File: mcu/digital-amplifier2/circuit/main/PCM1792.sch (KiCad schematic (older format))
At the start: 16 parts, among them U12 PCM1792A

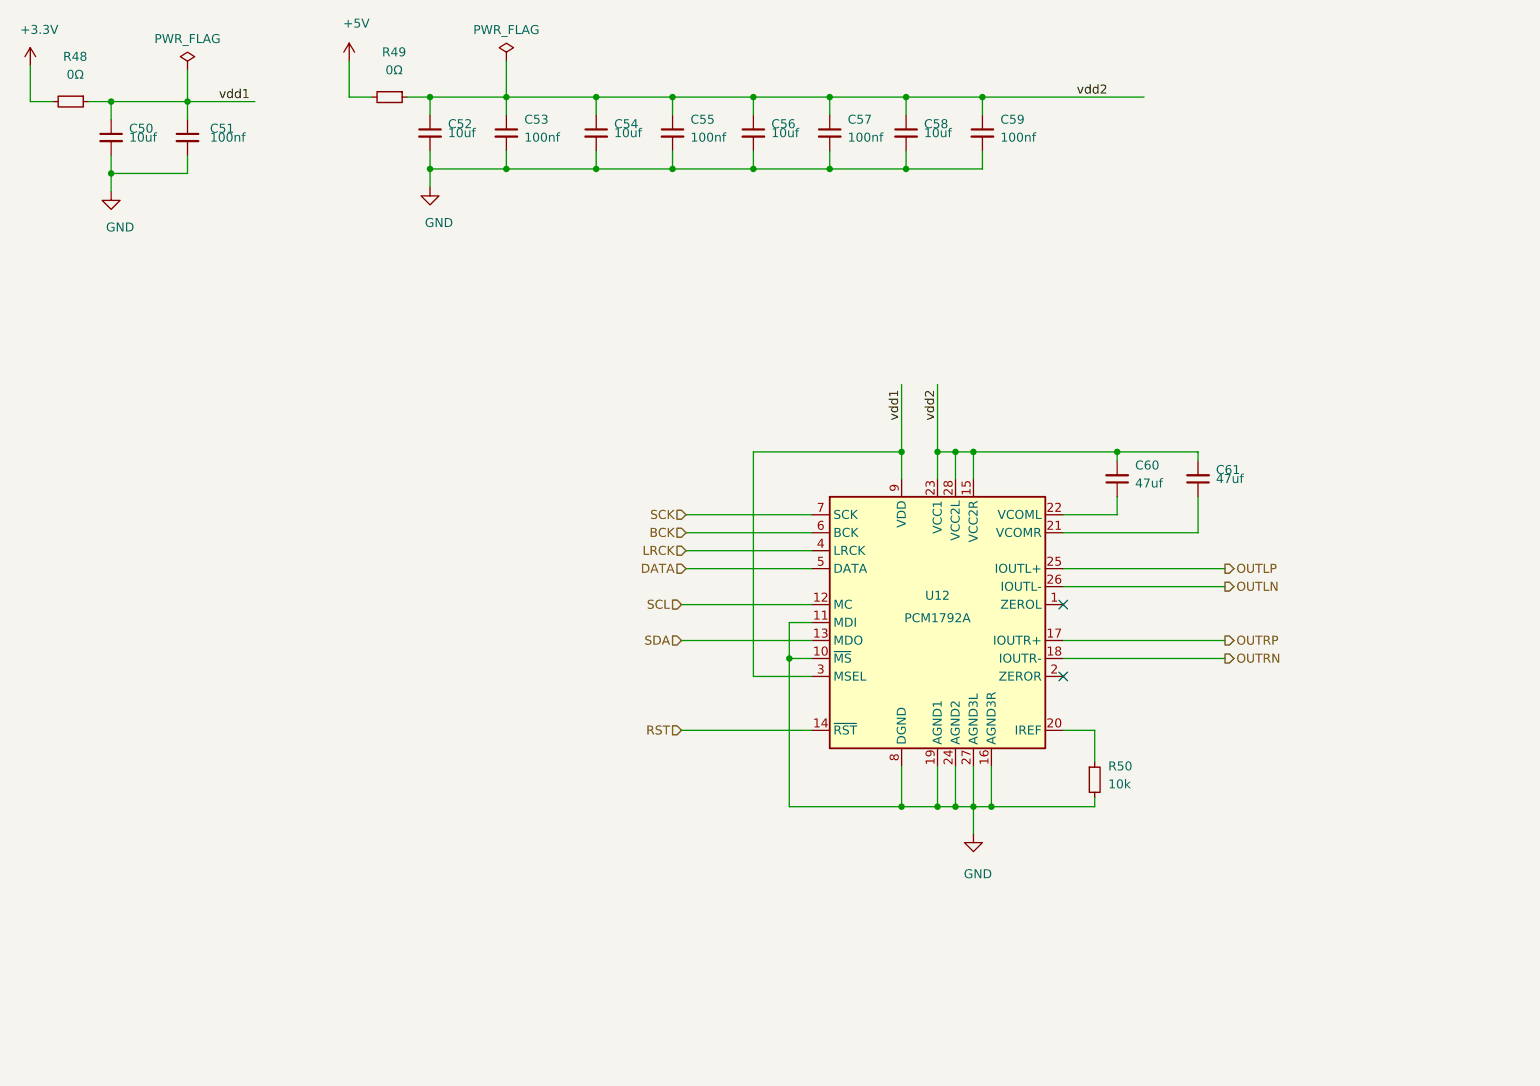
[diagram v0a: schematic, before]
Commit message: v5
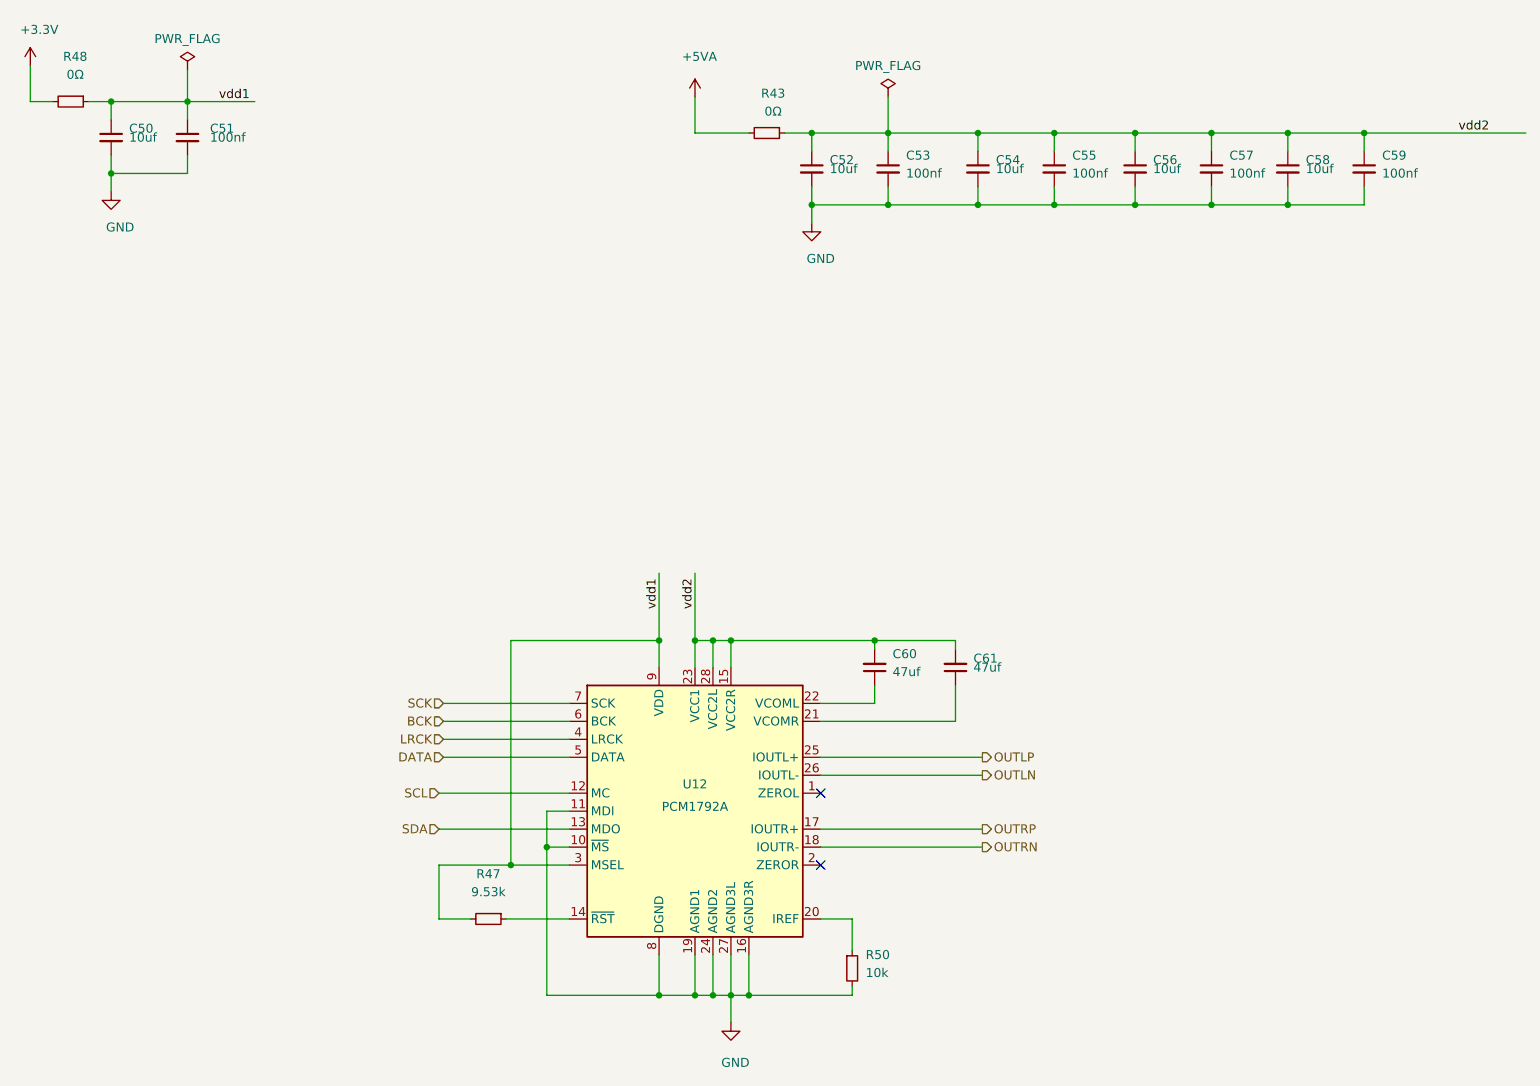
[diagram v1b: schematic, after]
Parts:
- removed R49: 0Ω, Resistor_SMD:R_0805_2012Metric, symbol Device:R_Small
- added R43: 0Ω, Resistor_SMD:R_0805_2012Metric, symbol Device:R_Small
- added R47: 9.53k, Resistor_SMD:R_0805_2012Metric, symbol Device:R_Small
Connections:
- net labels added: +5VA
- net labels removed: +5V, RST
- wire segments 97 -> 100
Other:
- moved on the sheet: C52, C53, C54, C55, C56, C57, C58, C59, C60, C61, R50, U12
